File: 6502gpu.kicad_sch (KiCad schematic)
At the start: 6 parts, among them J1 DE15_Receptacle_HighDensity, J2 Conn_01x14, J3 Conn_01x08, J4 Conn_01x01, J5 Conn_01x02, U32 74HC00

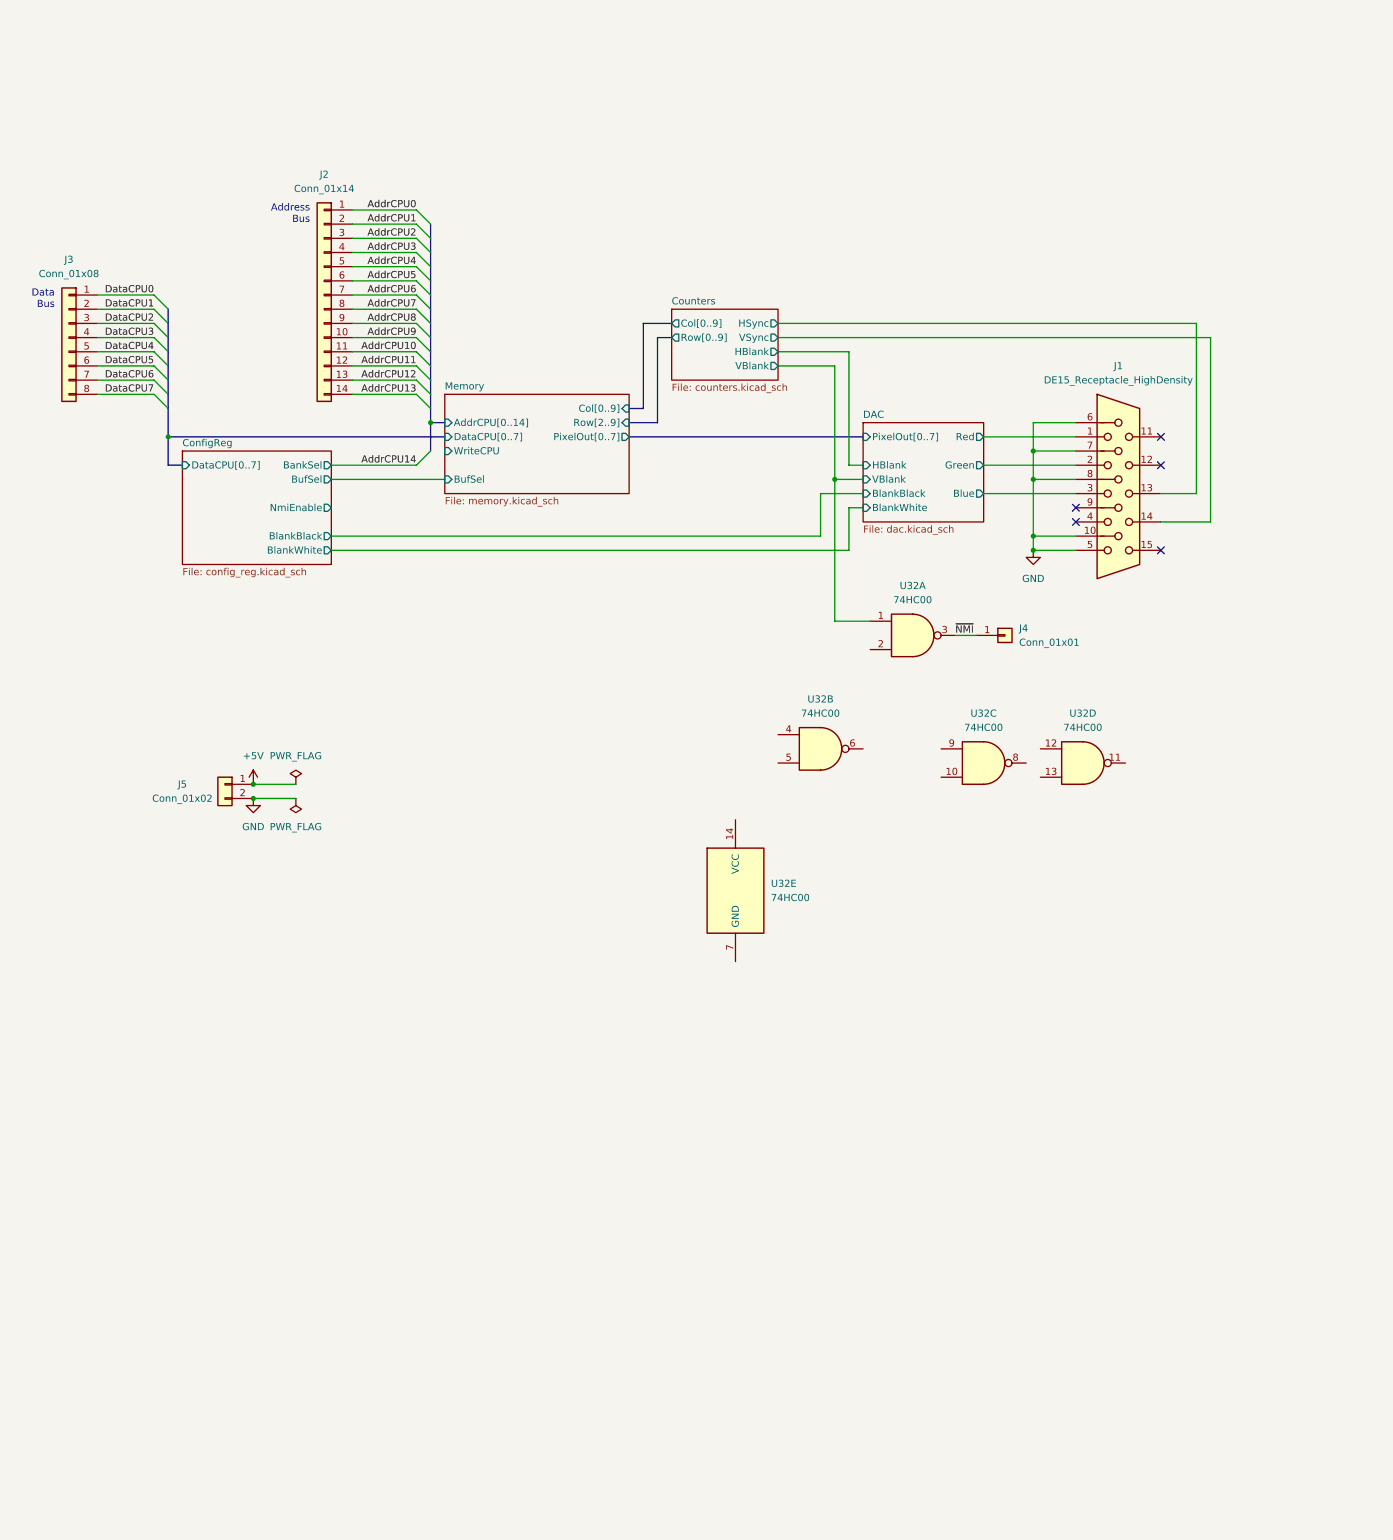
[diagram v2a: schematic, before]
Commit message: work on DAC
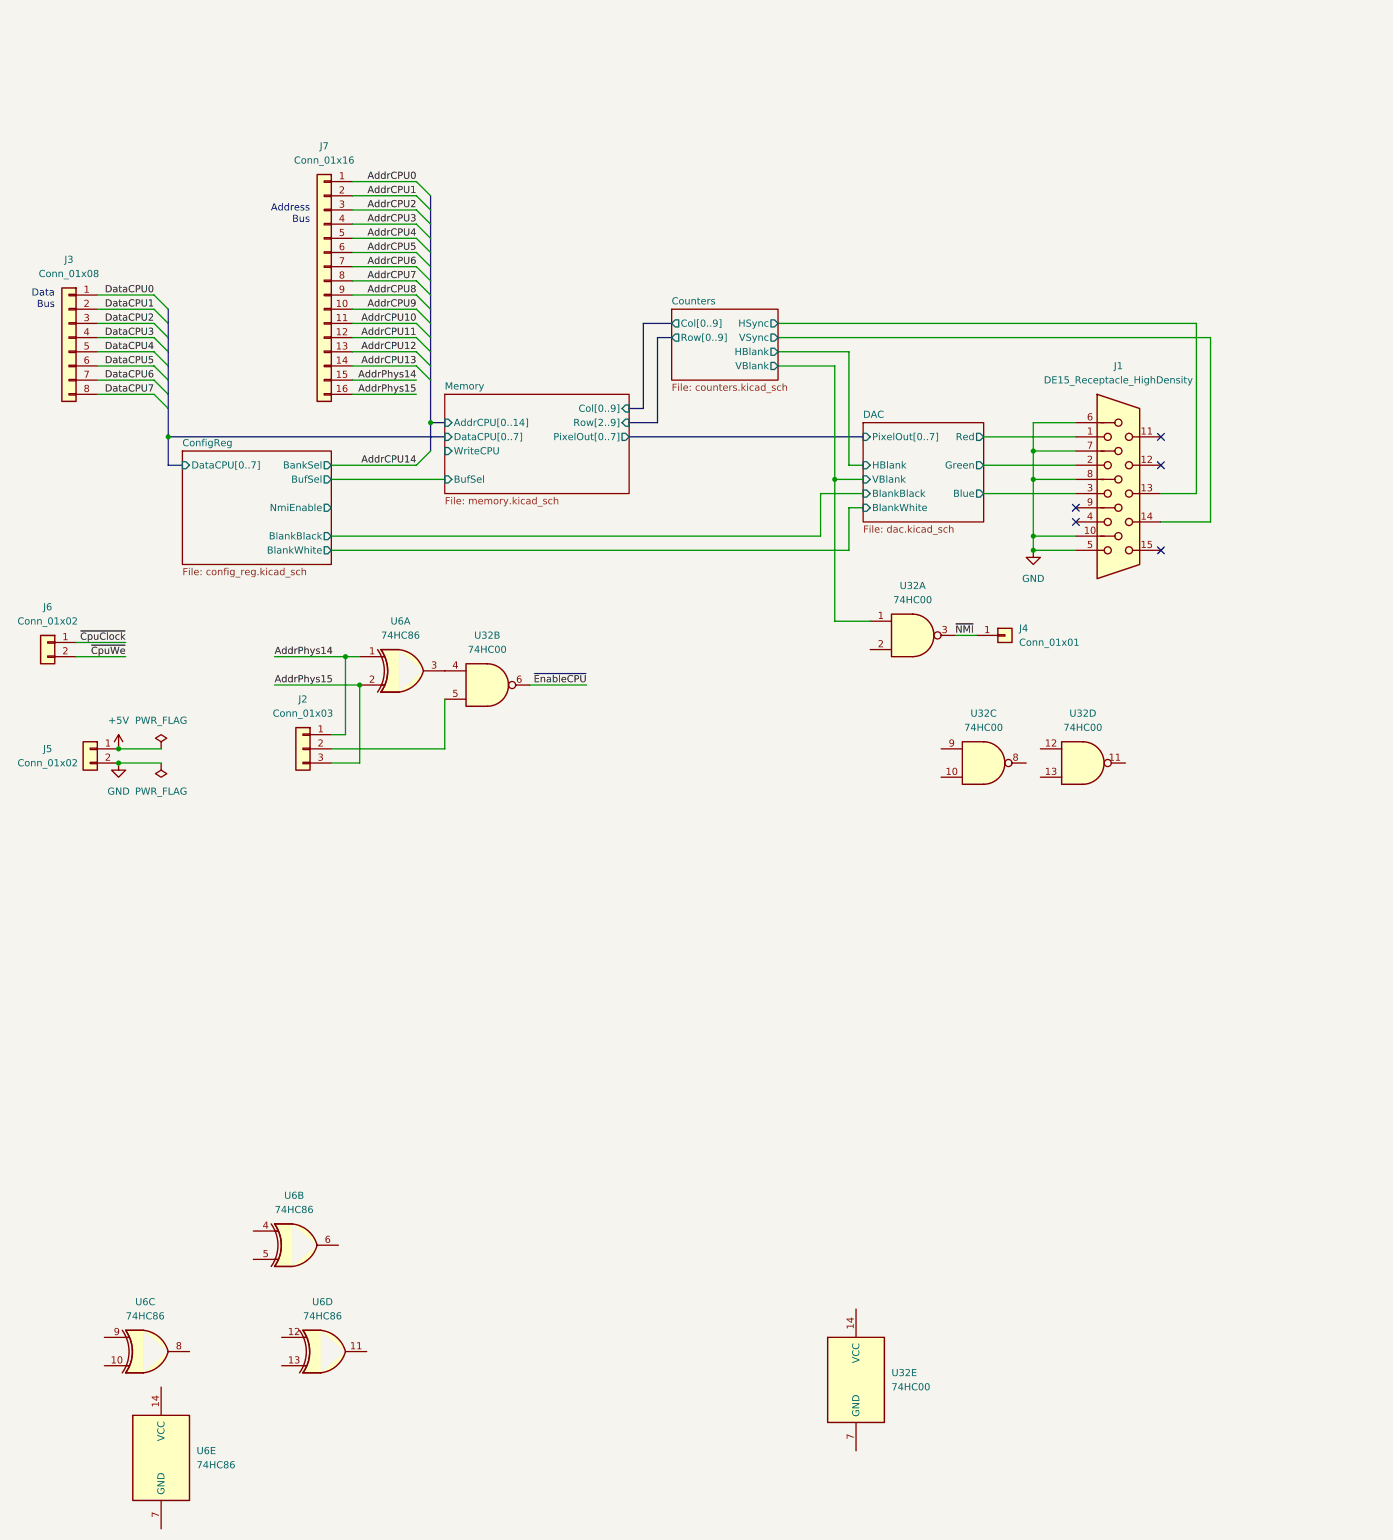
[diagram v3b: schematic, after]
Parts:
- removed J2: Conn_01x14, symbol Connector_Generic:Conn_01x14
- added J2: Conn_01x03, symbol Connector_Generic:Conn_01x03
- added J6: Conn_01x02, symbol Connector_Generic:Conn_01x02
- added J7: Conn_01x16, symbol Connector_Generic:Conn_01x16
- added U6: 74HC86, symbol 74xx:74HC86
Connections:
- net AddrCPU0: now also J7.1 (Pin_1)
- net AddrCPU1: now also J7.2 (Pin_2)
- net AddrCPU10: now also J7.11 (Pin_11)
- net AddrCPU11: now also J7.12 (Pin_12)
- net AddrCPU12: now also J7.13 (Pin_13)
- net AddrCPU13: now also J7.14 (Pin_14)
- net AddrCPU2: now also J7.3 (Pin_3)
- net AddrCPU3: now also J7.4 (Pin_4)
- net AddrCPU4: now also J7.5 (Pin_5)
- net AddrCPU5: now also J7.6 (Pin_6)
- net AddrCPU6: now also J7.7 (Pin_7)
- net AddrCPU7: now also J7.8 (Pin_8)
- net AddrCPU8: now also J7.9 (Pin_9)
- net AddrCPU9: now also J7.10 (Pin_10)
- net at U32.4: now also U6.3
- net at U32.5: now also J2.2 (Pin_2)
- net ~{EnableCPU}: now reaches U32.6
- new net AddrPhys14: J2.1 (Pin_1), J7.15 (Pin_15), U6.1
- new net AddrPhys15: J2.3 (Pin_3), J7.16 (Pin_16), U6.2
- new net ~{CpuClock}: J6.1 (Pin_1)
- new net ~{CpuWe}: J6.2 (Pin_2)
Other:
- moved on the sheet: J5, U32B, U32E
